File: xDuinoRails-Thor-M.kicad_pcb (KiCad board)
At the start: 6 copper layers, 30 x 20.1 mm, 46 parts, among them J701 Conn_02x11_Odd_Even, Q501 S8050, Q601 S8550, Q602 S8550, Q604 S8050, Q901 BSS138, Q902 BSS138, U1101 MOUDLE-SEEEDUINO-XIAO, U201 HT75xx-1-SOT89, U801 BDR6133

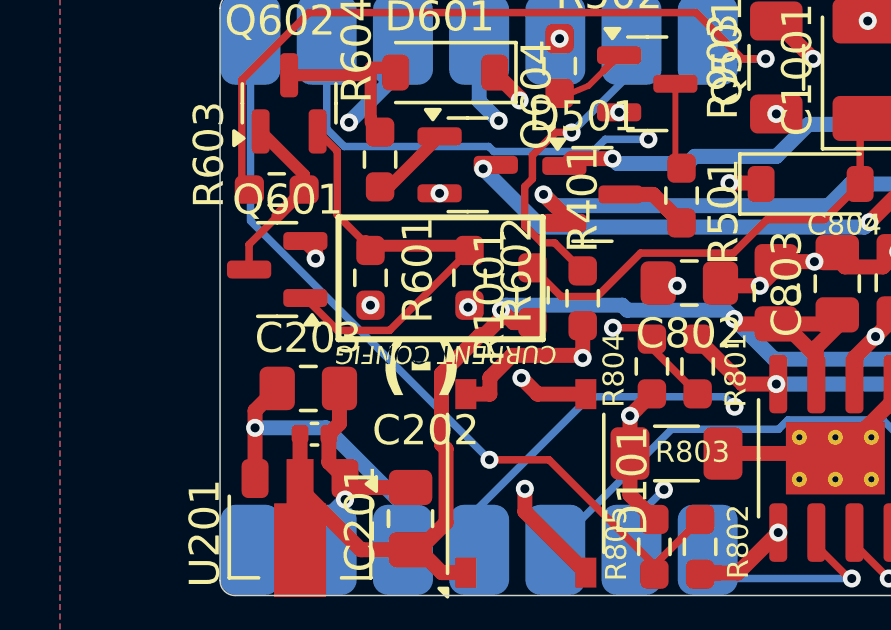
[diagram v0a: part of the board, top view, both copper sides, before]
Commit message: Fix - 3D model and some silkscreen
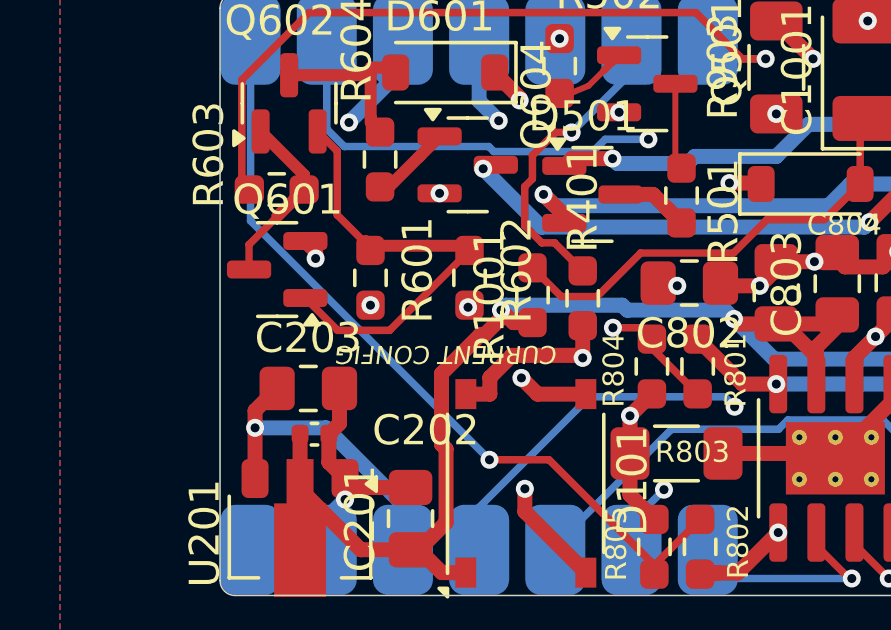
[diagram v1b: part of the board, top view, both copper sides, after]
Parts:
- U801: footprint Package_SO:SOIC-8-1EP_3.9x4.9mm_P1.27mm_EP2.41x3.3mm_ThermalVias -> xDuinoRail:SOIC-8-1EP_3.9x4.9mm_P1.27mm_EP2.41x3.3mm_ThermalVias
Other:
- board text removed: "(-)"
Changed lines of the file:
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@@
 		)
 	)
-	(footprint "Package_SO:SOIC-8-1EP_3.9x4.9mm_P1.27mm_EP2.41x3.3mm_ThermalVias"
+	(footprint "xDuinoRail:SOIC-8-1EP_3.9x4.9mm_P1.27mm_EP2.41x3.3mm_ThermalVias"
 		(layer "F.Cu")
 		(at 163.513 104.902 -90)
@@
 		(tags "SOIC SO")
 		(property "Reference" "U801"
-			(at 0 -3.4 90)
+			(at 0 -3.4 -90)
 			(layer "F.SilkS")
 			(effects
@@
 		)
 		(property "Value" "BDR6133"
-			(at -0.416 0.191 90)
+			(at 0 3.4 -90)
 			(layer "F.Fab")
 			(effects
@@
 			)
 		)
-		(property "Footprint" "Package_SO:SOIC-8-1EP_3.9x4.9mm_P1.27mm_EP2.41x3.3mm_ThermalVias"
-			(at 0 0 90)
+		(property "Footprint" "xDuinoRail:SOIC-8-1EP_3.9x4.9mm_P1.27mm_EP2.41x3.3mm_ThermalVias"
+			(at 0 0 -90)
 			(layer "F.Fab")
 			(hide yes)
@@
 		)
 		(property "Datasheet" ""
-			(at 0 0 90)
+			(at 0 0 -90)
 			(layer "F.Fab")
 			(hide yes)
@@
 		)
 		(property "Description" ""
-			(at 0 0 90)
+			(at 0 0 -90)
 			(layer "F.Fab")
 			(hide yes)
@@
 		(attr smd)
 		(fp_line
-			(start 0 2.559999)
+			(start 0 2.56)
 			(end -1.95 2.56)
 			(stroke
@@
 		)
 		(fp_line
-			(start 0 2.559999)
+			(start 0 2.56)
 			(end 1.95 2.56)
 			(stroke
@@
 		)
 		(fp_line
-			(start 0 -2.559999)
+			(start 0 -2.56)
 			(end -1.95 -2.56)
 			(stroke
@@
 		)
 		(fp_line
-			(start 0 -2.559999)
+			(start 0 -2.56)
 			(end 1.95 -2.56)
 			(stroke
@@
 		(fp_poly
 			(pts
-				(xy -2.7 -2.465) (xy -2.939999 -2.795) (xy -2.46 -2.795) (xy -2.7 -2.465)
+				(xy -2.7 -2.465) (xy -2.94 -2.795) (xy -2.46 -2.795) (xy -2.7 -2.465)
 			)
 			(stroke
@@
 		(fp_line
 			(start -1.95 -1.475)
-			(end -0.975 -2.450001)
+			(end -0.975 -2.45)
 			(stroke
 				(width 0.1)
@@
 		)
 		(fp_line
-			(start 1.95 -2.45)
-			(end 1.95 2.45)
+			(start -0.975 -2.45)
+			(end 1.95 -2.45)
 			(stroke
 				(width 0.1)
@@
 		)
 		(fp_line
-			(start -0.975 -2.450001)
-			(end 1.95 -2.45)
+			(start 1.95 -2.45)
+			(end 1.95 2.45)
 			(stroke
 				(width 0.1)
@@
 		)
 		(fp_text user "${REFERENCE}"
-			(at 0 0 90)
+			(at 0 0 -90)
 			(layer "F.Fab")
 			(effects
@@
 			(drill 0.2)
 			(property pad_prop_heatsink)
-			(layers "*.Cu" "In5.Cu" "In6.Cu" "In7.Cu" "In8.Cu" "In9.Cu" "In10.Cu"
-				"In11.Cu" "In12.Cu" "In13.Cu" "In14.Cu" "In15.Cu" "In16.Cu" "In17.Cu"
-				"In18.Cu" "In19.Cu" "In20.Cu" "In21.Cu" "In22.Cu" "In23.Cu" "In24.Cu"
-				"In25.Cu" "In26.Cu" "In27.Cu" "In28.Cu" "In29.Cu" "In30.Cu"
-			)
+			(layers "*.Cu")
 			(remove_unused_layers no)
 			(net 39 "PGND")
@@
 			(drill 0.2)
 			(property pad_prop_heatsink)
-			(layers "*.Cu" "In5.Cu" "In6.Cu" "In7.Cu" "In8.Cu" "In9.Cu" "In10.Cu"
-				"In11.Cu" "In12.Cu" "In13.Cu" "In14.Cu" "In15.Cu" "In16.Cu" "In17.Cu"
-				"In18.Cu" "In19.Cu" "In20.Cu" "In21.Cu" "In22.Cu" "In23.Cu" "In24.Cu"
-				"In25.Cu" "In26.Cu" "In27.Cu" "In28.Cu" "In29.Cu" "In30.Cu"
-			)
+			(layers "*.Cu")
 			(remove_unused_layers no)
 			(net 39 "PGND")
@@
 			(drill 0.2)
 			(property pad_prop_heatsink)
-			(layers "*.Cu" "In5.Cu" "In6.Cu" "In7.Cu" "In8.Cu" "In9.Cu" "In10.Cu"
-				"In11.Cu" "In12.Cu" "In13.Cu" "In14.Cu" "In15.Cu" "In16.Cu" "In17.Cu"
-				"In18.Cu" "In19.Cu" "In20.Cu" "In21.Cu" "In22.Cu" "In23.Cu" "In24.Cu"
-				"In25.Cu" "In26.Cu" "In27.Cu" "In28.Cu" "In29.Cu" "In30.Cu"
-			)
+			(layers "*.Cu")
 			(remove_unused_layers no)
 			(net 39 "PGND")
@@
 			(drill 0.2)
 			(property pad_prop_heatsink)
-			(layers "*.Cu" "In5.Cu" "In6.Cu" "In7.Cu" "In8.Cu" "In9.Cu" "In10.Cu"
-				"In11.Cu" "In12.Cu" "In13.Cu" "In14.Cu" "In15.Cu" "In16.Cu" "In17.Cu"
-				"In18.Cu" "In19.Cu" "In20.Cu" "In21.Cu" "In22.Cu" "In23.Cu" "In24.Cu"
-				"In25.Cu" "In26.Cu" "In27.Cu" "In28.Cu" "In29.Cu" "In30.Cu"
-			)
+			(layers "*.Cu")
 			(remove_unused_layers no)
 			(net 39 "PGND")
@@
 			(drill 0.2)
 			(property pad_prop_heatsink)
-			(layers "*.Cu" "In5.Cu" "In6.Cu" "In7.Cu" "In8.Cu" "In9.Cu" "In10.Cu"
-				"In11.Cu" "In12.Cu" "In13.Cu" "In14.Cu" "In15.Cu" "In16.Cu" "In17.Cu"
-				"In18.Cu" "In19.Cu" "In20.Cu" "In21.Cu" "In22.Cu" "In23.Cu" "In24.Cu"
-				"In25.Cu" "In26.Cu" "In27.Cu" "In28.Cu" "In29.Cu" "In30.Cu"
-			)
+			(layers "*.Cu")
 			(remove_unused_layers no)
 			(net 39 "PGND")
@@
 			(drill 0.2)
 			(property pad_prop_heatsink)
-			(layers "*.Cu" "In5.Cu" "In6.Cu" "In7.Cu" "In8.Cu" "In9.Cu" "In10.Cu"
-				"In11.Cu" "In12.Cu" "In13.Cu" "In14.Cu" "In15.Cu" "In16.Cu" "In17.Cu"
-				"In18.Cu" "In19.Cu" "In20.Cu" "In21.Cu" "In22.Cu" "In23.Cu" "In24.Cu"
-				"In25.Cu" "In26.Cu" "In27.Cu" "In28.Cu" "In29.Cu" "In30.Cu"
-			)
+			(layers "*.Cu")
 			(remove_unused_layers no)
 			(net 39 "PGND")
@@
 			(pintype "power_in")
 		)
-		(model "${KICAD8_3DMODEL_DIR}/Package_SO.3dshapes/SOIC-8-1EP_3.9x4.9mm_P1.27mm_EP2.41x3.3mm.wrl"
+		(model "${KICAD8_3DMODEL_DIR}/Package_SO.3dshapes/SOIC-8-1EP_3.9x4.9mm_P1.27mm_EP2.29x3mm.wrl"
 			(offset
 				(xyz 0 0 0)
@@
 			)
 		)
-		(property "OLI_ID" "100nF_0603"
+		(property "OLI_ID" "100nF_0805"
 			(at 0 0 90)
 			(unlocked yes)
@@
 		(fp_arc
 			(start -6.600468 10.499999)
-			(mid -7.949608 10.111768)
+			(mid -7.949609 10.111769)
 			(end -8.812892 9.00468)
 			(stroke
@@
 		(fp_arc
 			(start 8.804034 9.001464)
-			(mid 7.944327 10.107119)
+			(mid 7.944325 10.107118)
 			(end 6.6 10.499999)
 			(stroke
@@
 			(layer "B.SilkS")
 		)
-		(fp_poly
-			(pts
-				(xy -11 12) (xy 11 12) (xy 11 -11) (xy -11 -11)
-			)
+		(fp_rect
+			(start -11 12)
+			(end 11 -11)
 			(stroke
 				(width 0.05)
@@
 		)
 		(pad "4" smd roundrect
-			(at -8.500001 0 270)
+			(at -8.5 0 270)
 			(size 3 2)
 			(layers "B.Cu" "B.Paste" "B.Mask")
@@
 		)
 		(pad "11" smd roundrect
-			(at 8.500001 0 270)
+			(at 8.5 0 270)
 			(size 3 2)
 			(layers "B.Cu" "B.Paste" "B.Mask")
@@
 			)
 		)
+		(model "${KIPRJMOD}/__lib/3d/SeeedStudio-XIAO_RP2040-v26.step"
+			(offset
+				(xyz 0 0 0)
+			)
+			(scale
+				(xyz 1 1 1)
+			)
+			(rotate
+				(xyz 0 0 0)
+			)
+		)
 	)
 	(footprint "TestPoint:TestPoint_Pad_D1.0mm"
@@
 		(layer "B.SilkS")
 	)
-	(gr_poly
-		(pts
-			(xy 153.756699 96.869666) (xy 153.756701 100.933665) (xy 146.9495 100.933665) (xy 146.9495 96.869665)
-		)
-		(stroke
-			(width 0.2)
-			(type default)
-		)
-		(fill none)
-		(layer "F.SilkS")
-	)
 	(gr_line
 		(start 143.502 89.402)
@@
 		)
 	)
-	(gr_text "(-)"
-		(at 148.336 101.0495 180)
-		(layer "F.SilkS")
-		(effects
-			(font
-				(size 1.5 1.5)
-				(thickness 0.3)
-				(bold yes)
-			)
-			(justify left bottom mirror)
-		)
-	)
 	(gr_text "Fehlender PIN"
 		(at 170.688 109.22 0)
@@
 		)
 	)
+	(group "subpcb_Stammblatt/rails_power_dc-dc-ldo-3v3_100mA"
+		(members "2495a32d-55d5-45c7-bf0d-90cec6114754" "8e28e822-f441-4a15-be24-b48dd8eb495f"
+			"f9515013-ffaf-46c4-ab7f-0578365a6d72"
+		)
+	)
 	(group "subpcb_Stammblatt/c9229de7/rails-signal-acknowledge_dcc"
 		(members "4c5602bf-903a-4ddb-8536-de0387f532e7" "507af063-49e9-4d2d-8016-8e7985a9710e"
@@
 		)
 	)
-	(group "subpcb_Stammblatt/rails_power_dc-dc-ldo-3v3_100mA"
-		(members "2495a32d-55d5-45c7-bf0d-90cec6114754" "8e28e822-f441-4a15-be24-b48dd8eb495f"
-			"f0e60a2e-b953-45e2-a762-24d2fcbf639e" "f9515013-ffaf-46c4-ab7f-0578365a6d72"
-		)
-	)
 	(group "subpcb_Stammblatt/c9229de7/rails_signal_feedback_dcc-railcom-8x50"
 		(members "16a319d4-62fd-400f-99ab-9c4439dc6ad6" "208636e3-d876-4511-90f1-8264a7ae489d"
 			"2632b471-c93b-4688-8365-79cd481cc3e8" "38a3be87-99bb-44d1-b52d-145a29fadfaa"
-			"4bb585cb-cc7d-4218-ab08-242a7052c194" "515018a4-f51e-4572-ba6b-e25c6693ea96"
-			"52c5a9b6-2cd8-4100-a4d3-4889c73e808a" "706dbf31-a91e-4c06-8680-1c9521f5667d"
-			"b876a4a8-a94f-404b-8d49-0ccdbbe68970" "e9b7c0d0-b788-44ec-a06f-fcc71b4ef725"
+			"515018a4-f51e-4572-ba6b-e25c6693ea96" "52c5a9b6-2cd8-4100-a4d3-4889c73e808a"
+			"706dbf31-a91e-4c06-8680-1c9521f5667d" "b876a4a8-a94f-404b-8d49-0ccdbbe68970"
+			"e9b7c0d0-b788-44ec-a06f-fcc71b4ef725"
 		)
 	)
